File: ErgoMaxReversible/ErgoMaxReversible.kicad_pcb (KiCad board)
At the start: 2 copper layers, 182.8 x 169.2 mm, 102 parts, among them J1 PJ-320A, K1 KEYSW, K10 KEYSW, K11 KEYSW, K12 KEYSW, K13 KEYSW, K14 KEYSW, K15 KEYSW, K16 KEYSW, K17 KEYSW, K18 KEYSW, K19 KEYSW, K2 KEYSW, K20 KEYSW, K21 KEYSW, K22 KEYSW, K23 KEYSW, K24 KEYSW, K25 KEYSW, K26 KEYSW, K27 KEYSW, K28 KEYSW, K29 KEYSW, K3 KEYSW, K30 KEYSW, K31 KEYSW, K32 KEYSW, K33 KEYSW, K34 KEYSW, K35 KEYSW, K36 KEYSW, K37 KEYSW, K38 KEYSW, K39 KEYSW, K4 KEYSW, K40 KEYSW, K41 KEYSW, K42 KEYSW, K43 KEYSW, K44 KEYSW, K5 KEYSW, K6 KEYSW, K7 KEYSW, K8 KEYSW, K9 KEYSW, U1 ProMicro

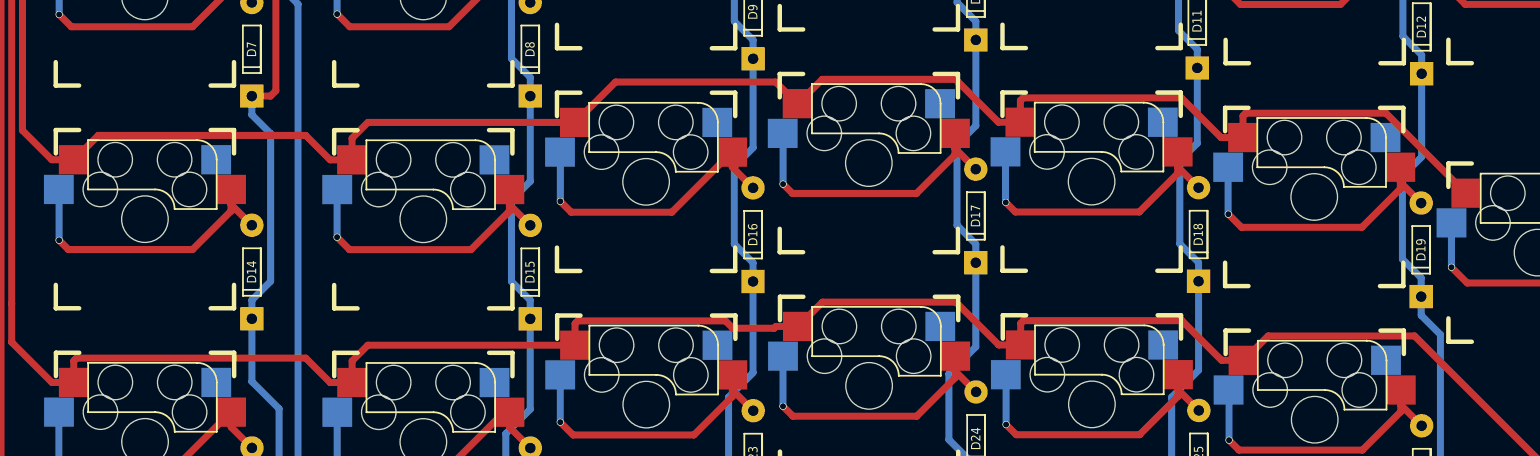
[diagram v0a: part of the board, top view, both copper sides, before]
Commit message: wiring again for reversible pcb
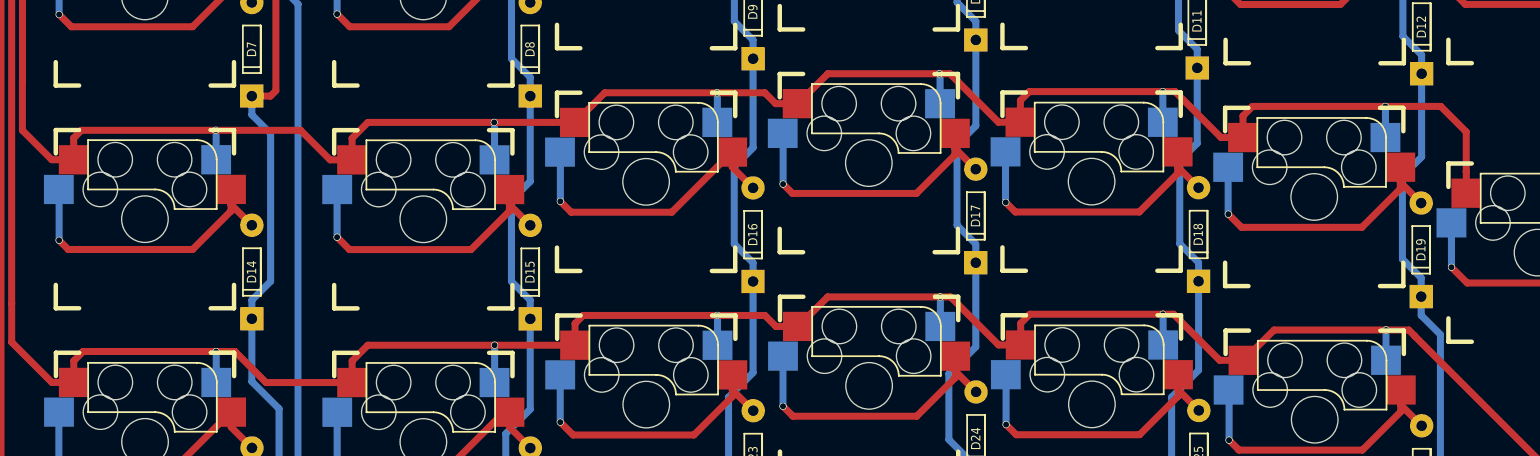
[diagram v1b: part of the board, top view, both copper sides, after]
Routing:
- net /Row2: track 180.2 -> 201.5 mm, vias 0 -> 6
- net /Row3: track 306.0 -> 324.1 mm, vias 1 -> 7
